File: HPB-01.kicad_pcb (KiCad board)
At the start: 2 copper layers, 60 x 27 mm, 55 parts, among them J1 USB_A, J4 USB_C_Receptacle_USB2.0, J5 Pad, J6 Pad, J7 Battery Pad, J8 Battery Pad, Q1 RU207C, Q4 RU20P7C, Q5 IRF7832, Q6 IRF7832, SW1 SW_Push, U1 S-8261ABJMD-G3JT2S, U2 IP5328P

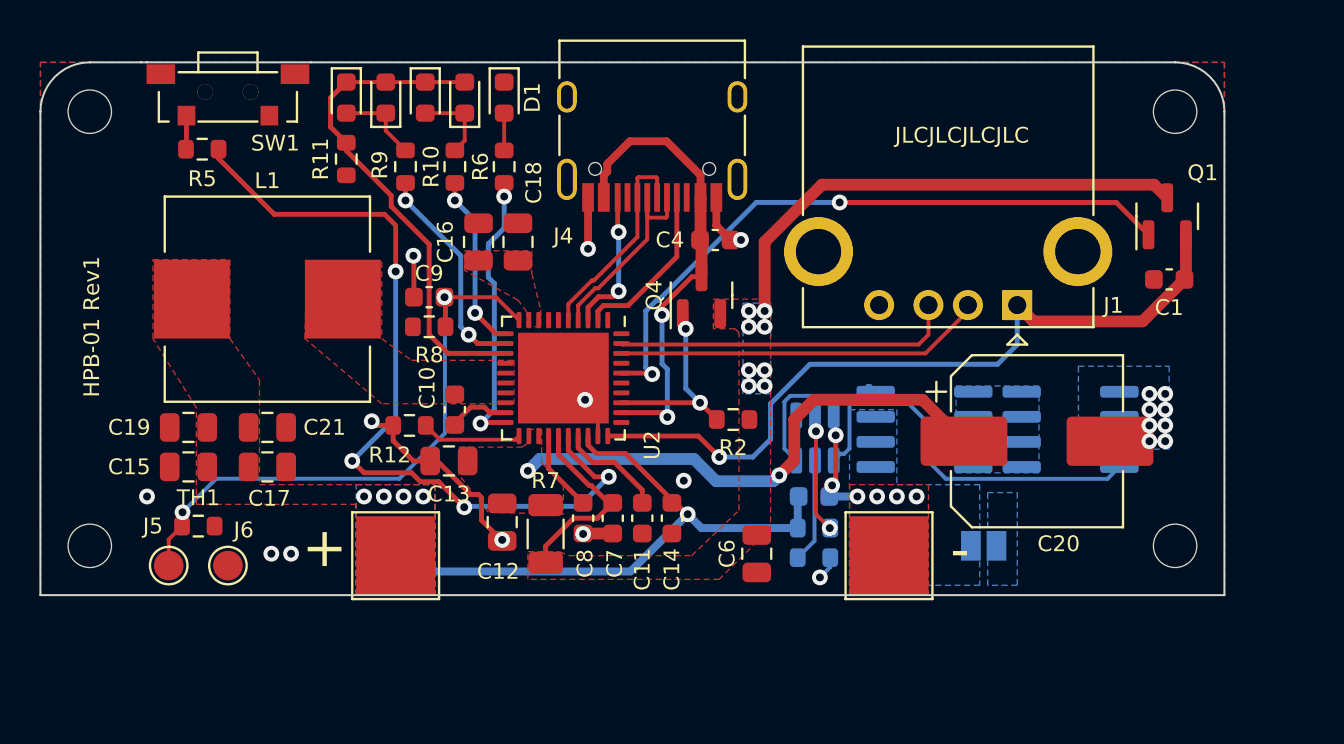
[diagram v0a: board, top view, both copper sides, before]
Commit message: Change the layout (bigger)
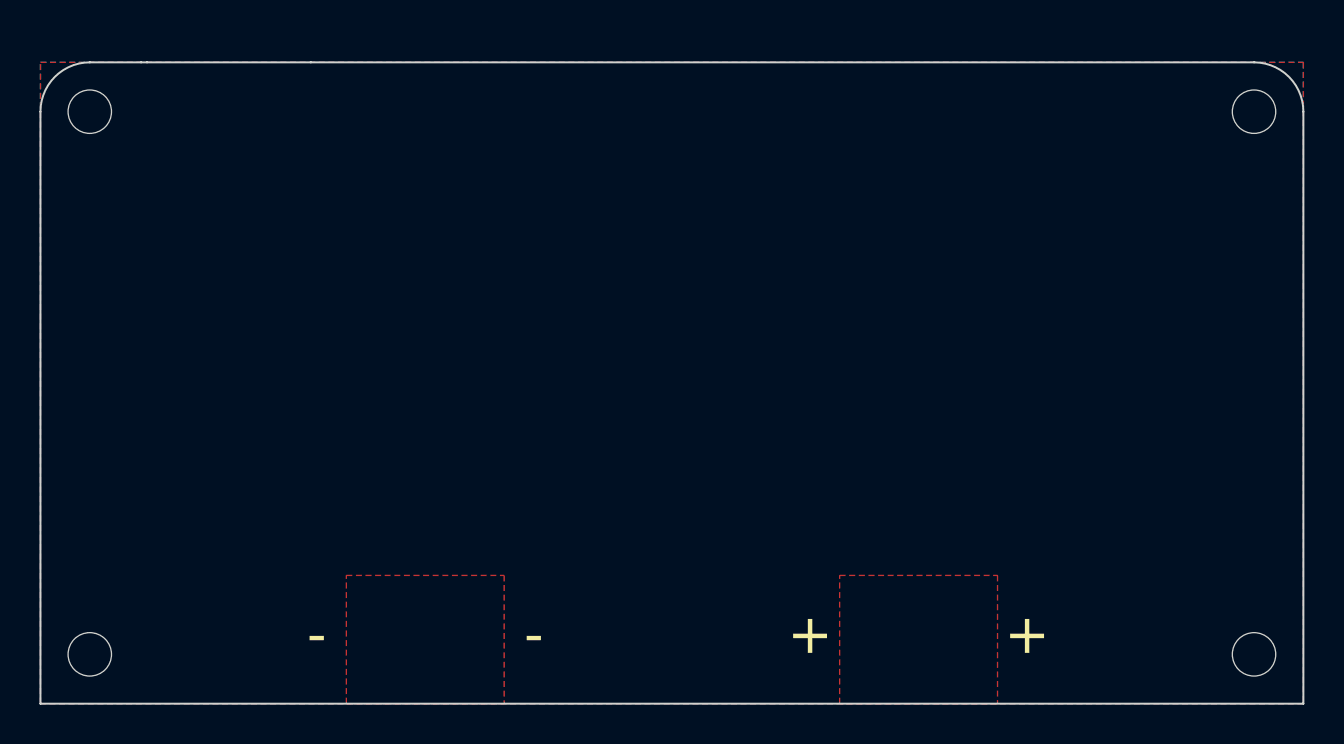
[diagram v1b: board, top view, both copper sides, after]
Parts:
- removed C1, C4: 10uF, Capacitor_SMD:C_0603_1608Metric
- removed C10, C5, C7, C8, C9: 100nF, Capacitor_SMD:C_0603_1608Metric
- removed C11, C14: 2.2uF, Capacitor_SMD:C_0603_1608Metric
- removed C12, C13, C15, C16, C17, C18, C19, C21, C6: 22uF, Capacitor_SMD:C_0805_2012Metric
- removed C20: 220uF, Capacitor_SMD:CP_Elec_8x10.5
- removed D1: GREEN, LED_SMD:LED_0603_1608Metric
- removed D2, D3, D4, D5: BLUE, LED_SMD:LED_0603_1608Metric
- removed J1: USB_A, Connector_USB:USB_A_CONNFLY_DS1095-WNR0
- removed J4: USB_C_Receptacle_USB2.0, Connector_USB:USB_C_Receptacle_HRO_TYPE-C-31-M-12
- removed J5, J6: Pad, TestPoint:TestPoint_Pad_D1.5mm
- removed J7, J8: Battery Pad, TestPoint:TestPoint_Pad_4.0x4.0mm
- removed JP1: SolderJumper_2_Open, Jumper:SolderJumper-2_P1.3mm_Open_Pad1.0x1.5mm
- removed L1: 2.2uH, Inductor_SMD:L_Wuerth_HCI-1050
- removed Q1: RU207C, Package_TO_SOT_SMD:SOT-23
- removed Q4: RU20P7C, Package_TO_SOT_SMD:SOT-23
- removed Q5, Q6: IRF7832, Package_SO:SOIC-8_3.9x4.9mm_P1.27mm
- removed R10, R6, R9: 100, Resistor_SMD:R_0603_1608Metric
- removed R11: NC, Resistor_SMD:R_0603_1608Metric
- removed R12: 114k, Resistor_SMD:R_0603_1608Metric
- removed R2: 10k, Resistor_SMD:R_0603_1608Metric
- removed R3: 2k, Resistor_SMD:R_0603_1608Metric
- removed R4: 470, Resistor_SMD:R_0603_1608Metric
- removed R5: 1k, Resistor_SMD:R_0603_1608Metric
- removed R7: 0.01, Resistor_SMD:R_1206_3216Metric
- removed R8: 82k(1%), Resistor_SMD:R_0603_1608Metric
- removed SW1: SW_Push, huconn-footprint:tact_switch 1TS002G-1300-3500-CT
- removed TH1: 100k@25C 4250K, Resistor_SMD:R_0603_1608Metric
- removed U1: S-8261ABJMD-G3JT2S, Package_TO_SOT_SMD:SOT-23-6
- removed U2: IP5328P, Package_DFN_QFN:QFN-40-1EP_6x6mm_P0.5mm_EP4.6x4.6mm
- moved H2 6.80 mm to (161.5, 100.0)
- moved H4 5.50 mm to (102.5, 100.0)
- moved H1 4.00 mm to (161.5, 72.5)
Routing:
- net /KEY: track 41.6 -> 0.00 mm, vias 4 -> 0
- net /VIN: track 38.6 -> 0.00 mm, vias 1 -> 0
- net /VMID: track 35.2 -> 0.00 mm, vias 8 -> 0
- net /VOUT1G: track 33.3 -> 0.00 mm, vias 2 -> 0
- net /VSP: track 30.7 -> 0.00 mm, vias 2 -> 0
- net /NTC: track 30.6 -> 0.00 mm, vias 2 -> 0
- net /VBAT: track 29.7 -> 0.00 mm, vias 5 -> 0
- net /L3: track 25.5 -> 0.00 mm
- net GND: track 24.4 -> 0.00 mm, vias 20 -> 0
- net /VBUS: track 23.6 -> 0.00 mm, vias 2 -> 0
- net /DFET: track 19.9 -> 0.00 mm
- net /USBA1_N: track 18.8 -> 0.00 mm
- net /USBA1_P: track 17.3 -> 0.00 mm
- net /LIGHT: track 14.2 -> 0.00 mm, vias 2 -> 0
- net /L2: track 11.1 -> 0.00 mm, vias 2 -> 0
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- removed copper zone on B.Cu, net /VBAT
- removed copper zone on B.Cu, net /VBAT-
- removed copper zone on B.Cu, net /VMID
- removed copper zone on F.Cu, net /VMID
- removed copper zone on F.Cu, net /VSP
- removed copper zone on F.Cu, net Net-(C10-Pad2)
- removed copper zone on B.Cu, net Net-(Q5-Pad5)
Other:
- board size 60 x 27 mm -> 64 x 32.5 mm
- board text removed: "HPB-01 Rev1"
- board text removed: "JLCJLCJLCJLC"
